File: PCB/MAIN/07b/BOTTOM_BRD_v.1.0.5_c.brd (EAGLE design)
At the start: 99.1 x 85.8 mm, 66 parts, among them Q1 SS8050, Q2 SS8050, Q4 TIP122, SW1 CS12ANW03, U1 ESP32-WROOM-32D, U2 L293D, U3 AP2112K-3.3, U4 CE8301

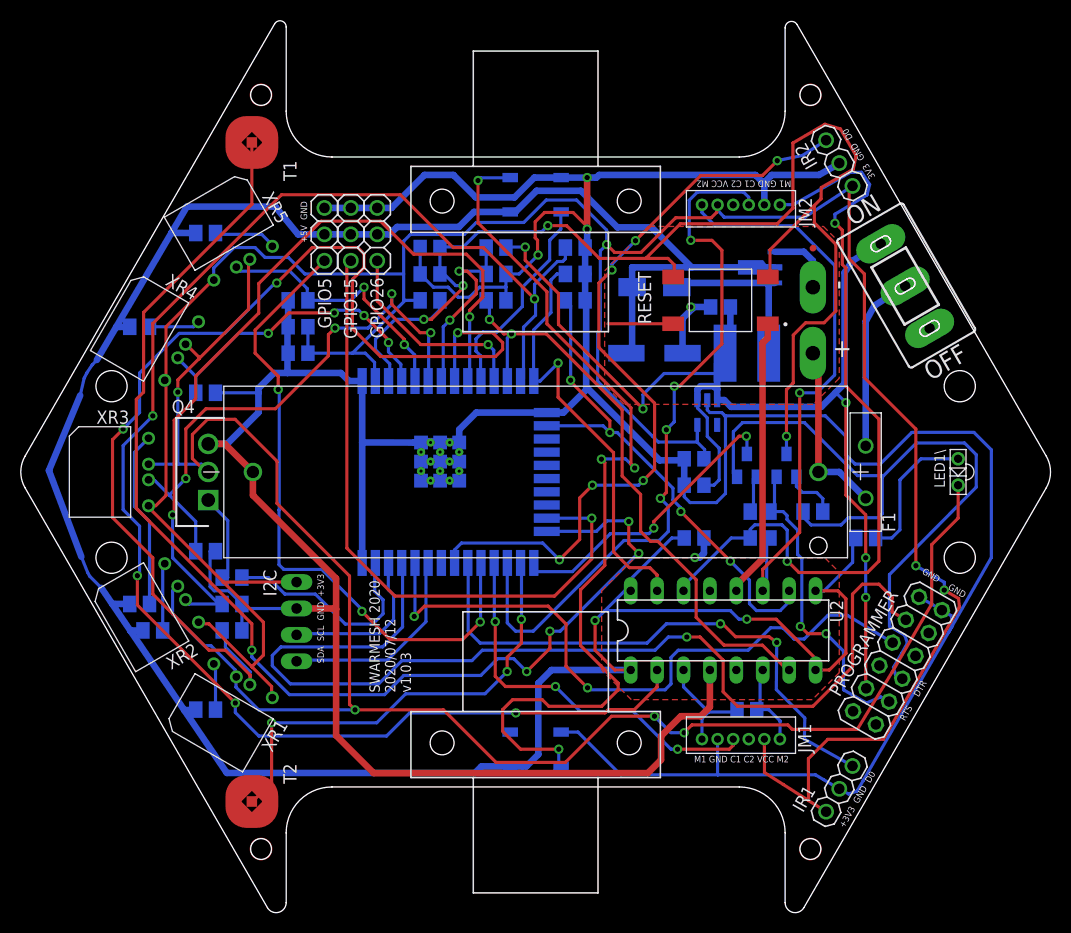
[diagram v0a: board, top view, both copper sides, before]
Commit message: Update BOTTOM_BRD_v.1.0.5_c.brd
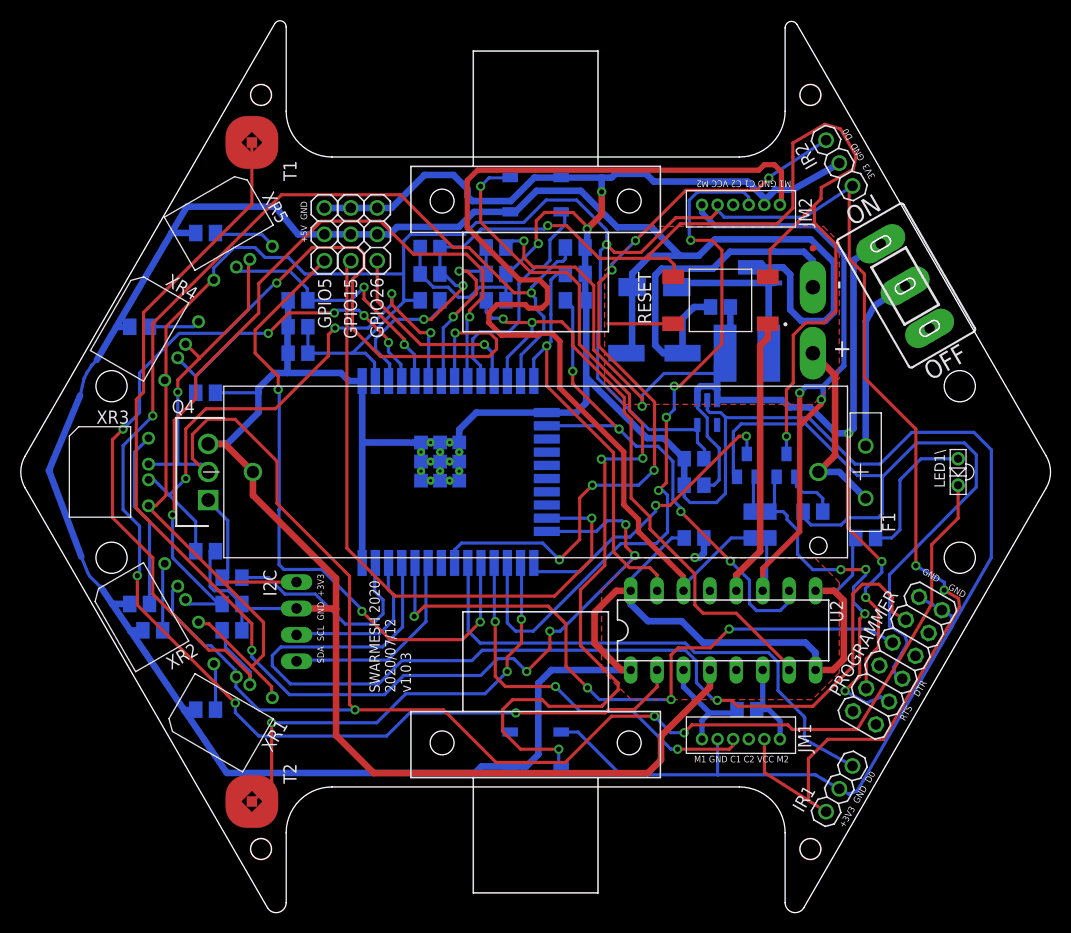
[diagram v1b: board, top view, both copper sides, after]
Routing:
- net M2A: track 76.2 -> 103.2 mm, vias 2 -> 0
- net +5V: track 257.0 -> 278.7 mm, vias 2 -> 0
- net GND: track 484.1 -> 505.6 mm, vias 5 -> 4
- net M2B: track 56.3 -> 62.9 mm, vias 1 -> 2
- net VCC: track 116.9 -> 122.6 mm
- net RTS: track 30.9 -> 36.0 mm, vias 2 -> 4
- net IR1: track 53.9 -> 51.4 mm, vias 2 -> 0
- net IO27: track 57.6 -> 59.9 mm
- net +3V3: track 275.1 -> 273.3 mm
- net LEDS: track 20.6 -> 22.5 mm
- net RXD: track 100.0 -> 98.4 mm
- net IO13: track 48.8 -> 50.4 mm
- net N$1: track 17.3 -> 18.6 mm
- net N$9: track 87.9 -> 89.1 mm
- net IO12: track 42.1 -> 41.2 mm
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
